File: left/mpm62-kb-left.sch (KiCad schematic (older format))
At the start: 68 parts, among them J1 Conn_01x04_Male, J2 Conn_01x02_Male, SW1 SW_Push, U1 ProMicro

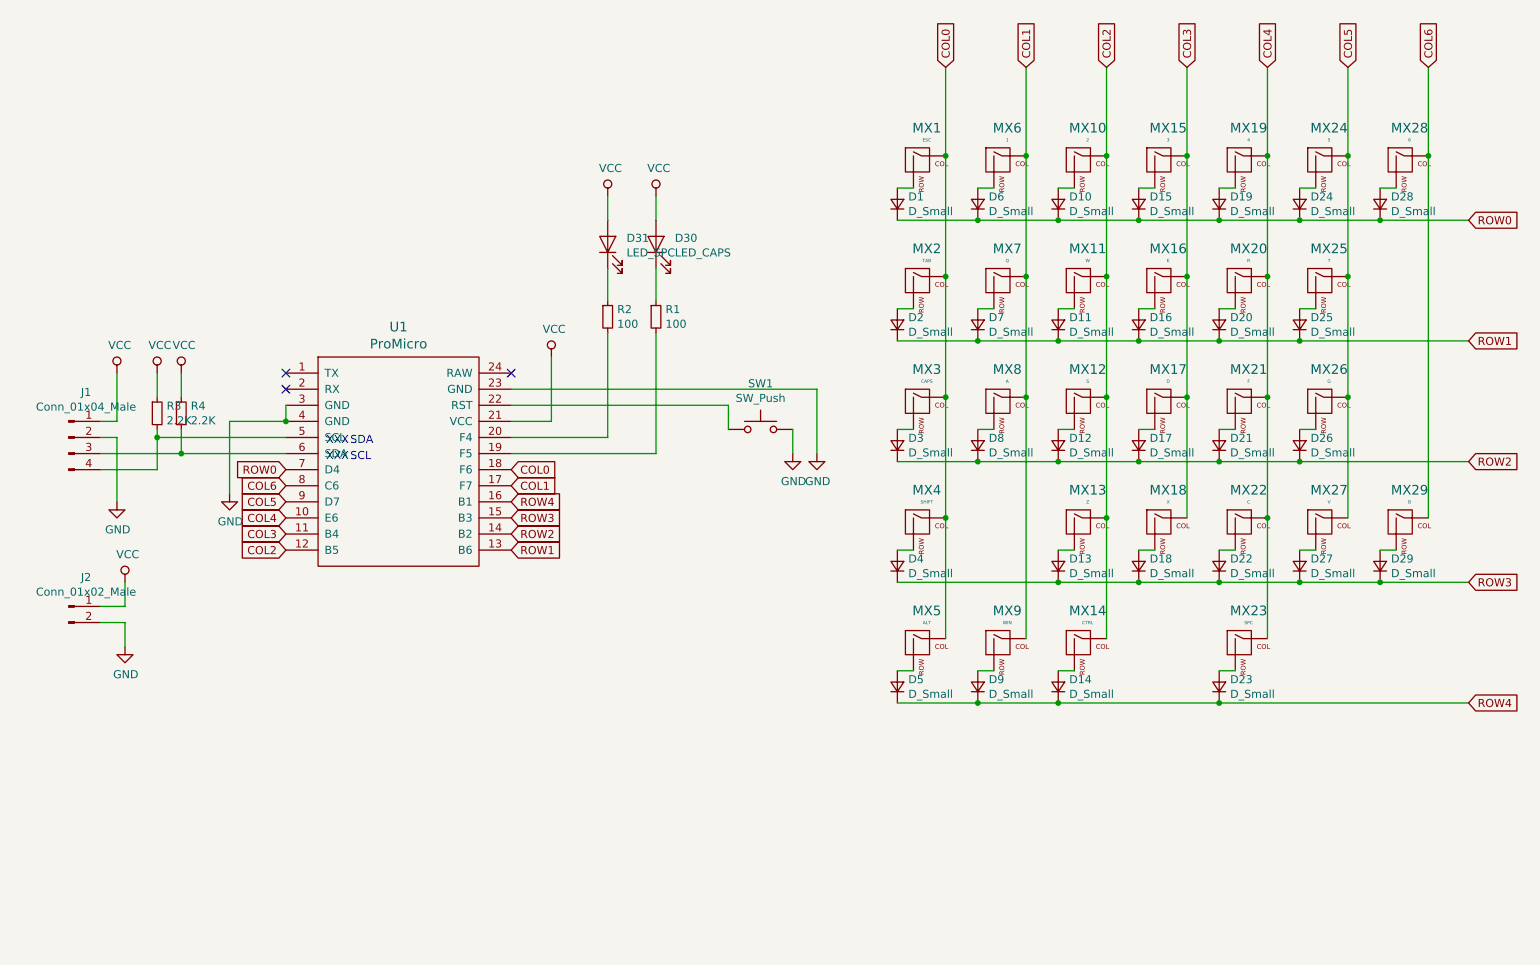
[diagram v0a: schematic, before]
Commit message: Final for b1t (board 1 thruhole) board
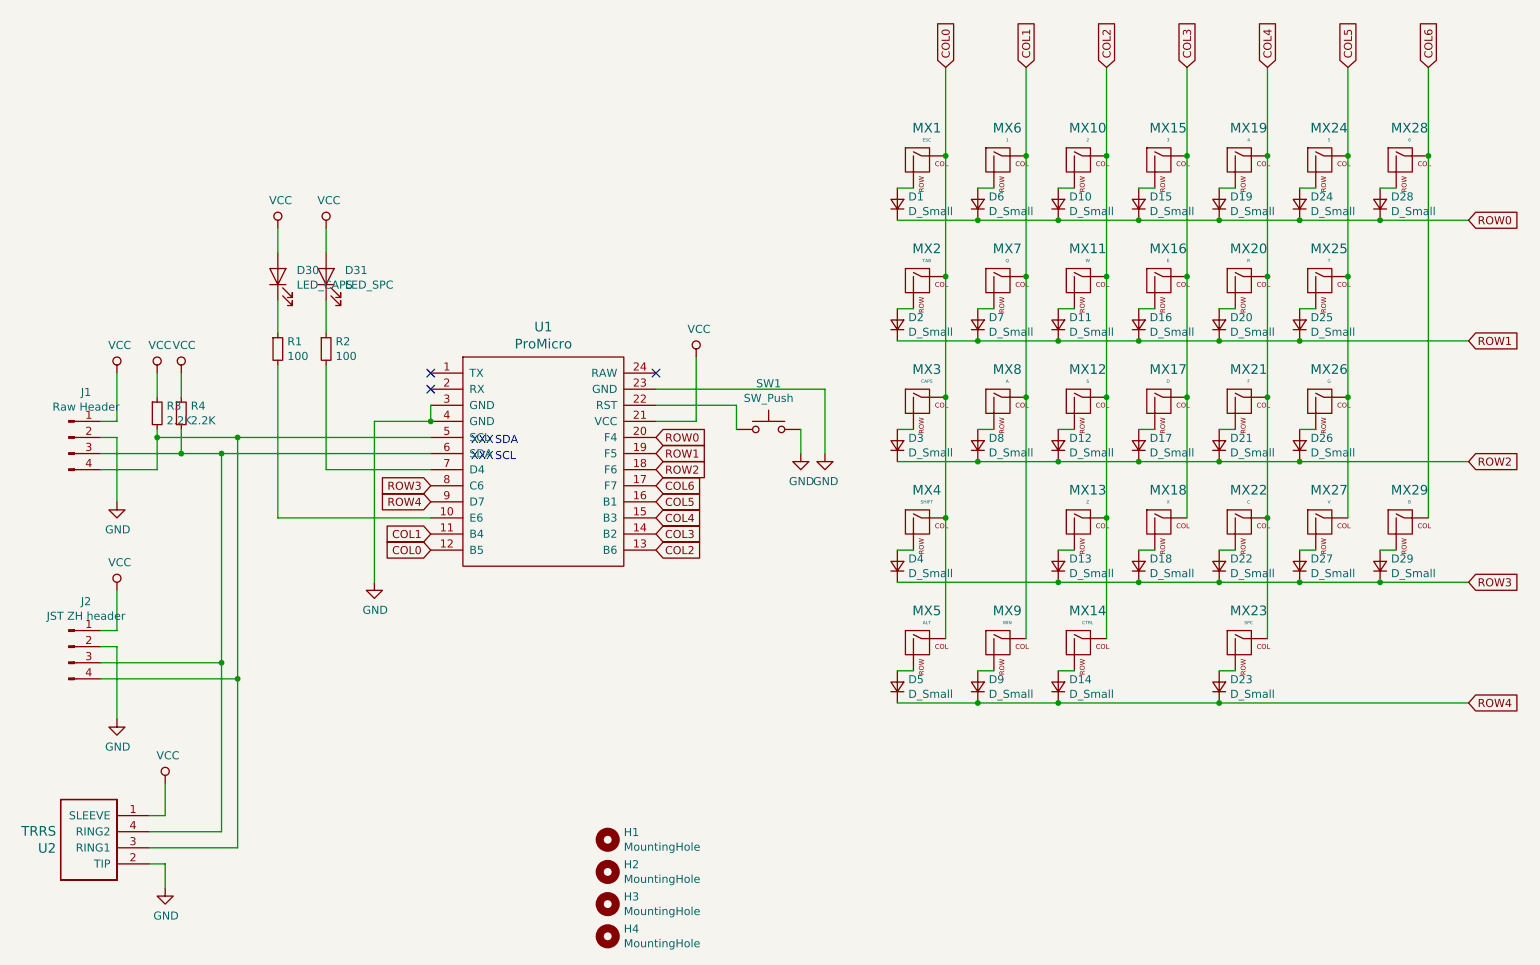
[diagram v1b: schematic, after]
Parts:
- removed J2: Conn_01x02_Male, Connector_PinHeader_2.54mm:PinHeader_1x02_P2.54mm_Vertical, symbol Connector:Conn_01x02_Male
- added H1, H2, H3, H4: MountingHole, MountingHole:MountingHole_2.2mm_M2_Pad, symbol Mechanical:MountingHole
- added J2: JST ZH header, MpmMisc:JST_ZH_B4B-ZR_1x04_P1.50mm_Vertical, symbol Connector:Conn_01x04_Male
- added U2: TRRS, Keebio-Parts:TRRS-PJ-320A, symbol keebio:TRRS
- J1: value Conn_01x04_Male -> Raw Header
- MX1, MX10, MX11, MX12, MX13, MX15, MX16, MX17, MX18, MX19, MX20, MX21, MX22, MX24, MX25, MX26, MX27, MX28, MX29, MX6, MX7, MX8: footprint MX_Alps_Hybrid:MX-1U-NoLED -> MX_Only:MXOnly-1U-NoLED
- MX14, MX5, MX9: footprint MX_Alps_Hybrid:MX-1.25U-NoLED -> MX_Only:MXOnly-1.25U-NoLED
- MX2: footprint MX_Alps_Hybrid:MX-1.5U-NoLED -> MX_Only:MXOnly-1.5U-NoLED
- MX23: footprint MX_Alps_Hybrid:MX-3U-ReversedStabilizers-NoLED -> MX_Only:MXOnly-3U-ReversedStabilizers-NoLED
- MX3: footprint MX_Alps_Hybrid:MX-1.75U-NoLED -> MX_Only:MXOnly-1.75U-NoLED
- MX4: footprint MX_Alps_Hybrid:MX-2.25U-NoLED -> MX_Only:MXOnly-2.25U-NoLED
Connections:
- net COL0: now also U1.12 (B5); no longer U1.18 (F6)
- net COL1: now also U1.11 (B4); no longer U1.17 (F7)
- net COL2: now also U1.13 (B6); no longer U1.12 (B5)
- net COL3: now also U1.14 (B2); no longer U1.11 (B4)
- net COL4: now also U1.15 (B3); no longer U1.10 (E6)
- net COL5: now also U1.16 (B1); no longer U1.9 (D7)
- net COL6: now also U1.17 (F7); no longer U1.8 (C6)
- net GND: now also J2.2 (Pin_2), U2.2 (TIP)
- net ROW0: now also U1.20 (F4); no longer U1.7 (D4)
- net ROW1: now also U1.19 (F5); no longer U1.13 (B6)
- net ROW2: now also U1.18 (F6); no longer U1.14 (B2)
- net ROW3: now also U1.8 (C6); no longer U1.15 (B3)
- net ROW4: now also U1.9 (D7); no longer U1.16 (B1)
- net VCC: now also J2.1 (Pin_1), U2.1 (SLEEVE)
- net at R1.2: now also U1.10 (E6); no longer U1.19 (F5)
- net at R2.2: now also U1.7 (D4); no longer U1.20 (F4)
- net at J1.4 (Pin_4), R3.2, U1.5 (SCL): now also J2.4 (Pin_4), U2.3 (RING1)
- net at J1.3 (Pin_3), R4.2, U1.6 (SDA): now also J2.3 (Pin_3), U2.4 (RING2)
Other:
- moved on the sheet: D30, D31, R1, R2, SW1, U1
